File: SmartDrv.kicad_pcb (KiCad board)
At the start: 4 copper layers, 60 x 60 mm, 97 parts, among them J1 Conn_01x04, J2 Conn_01x02, J3 Conn_01x02, J4 Conn_01x02, J5 Conn_01x02, J6 Conn_01x02, J7 Conn_01x03, Q1 BSC040N10NS5, Q2 BSC040N10NS5, Q3 BSC040N10NS5, Q4 BSC040N10NS5, Q5 PMOS, Q6 NPN, U1 IR2104, U2 IR2104, U3 AT32F423CBT7, U4 MCP6002-xSN, U5 TJA1051T, U6 AMS1117-5.0, U7 AP2112K-3.3, U8 L7812, U9 KF7.62-2P, Y1 Crystal_GND24

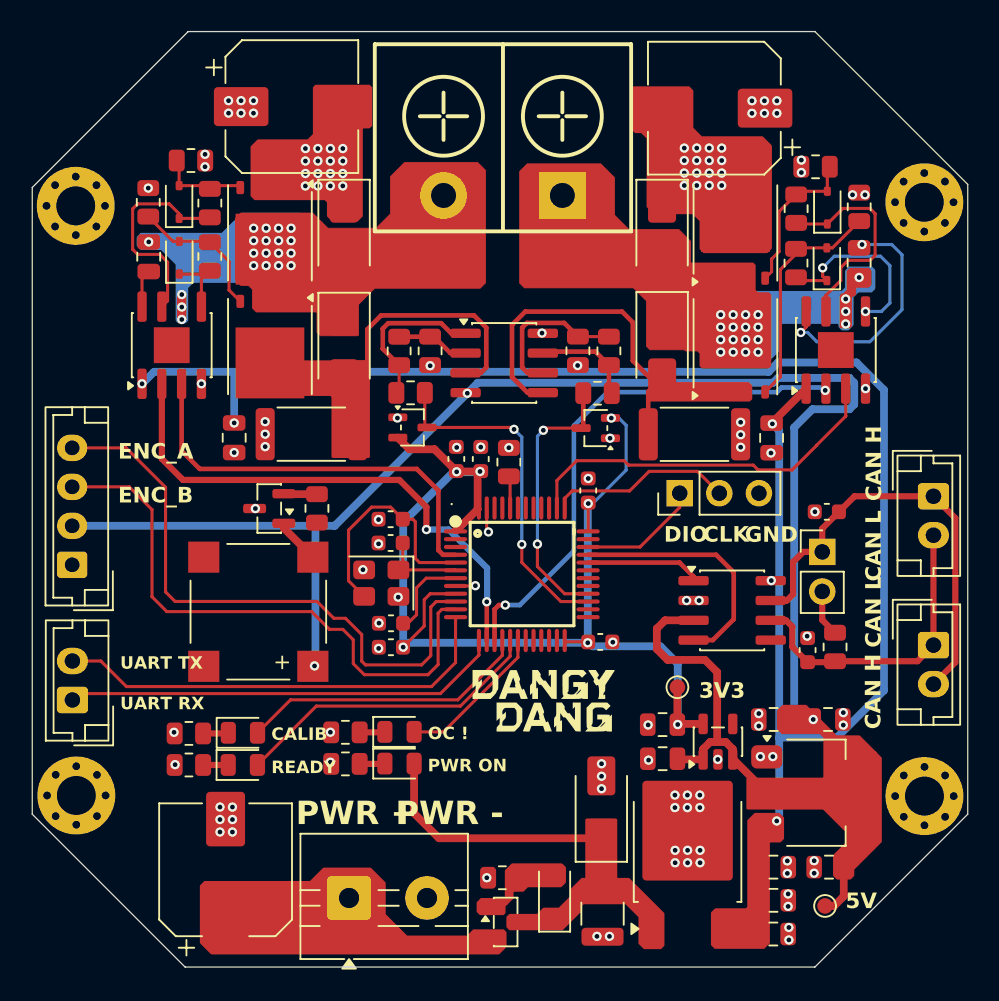
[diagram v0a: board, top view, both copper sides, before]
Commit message: Add files via upload
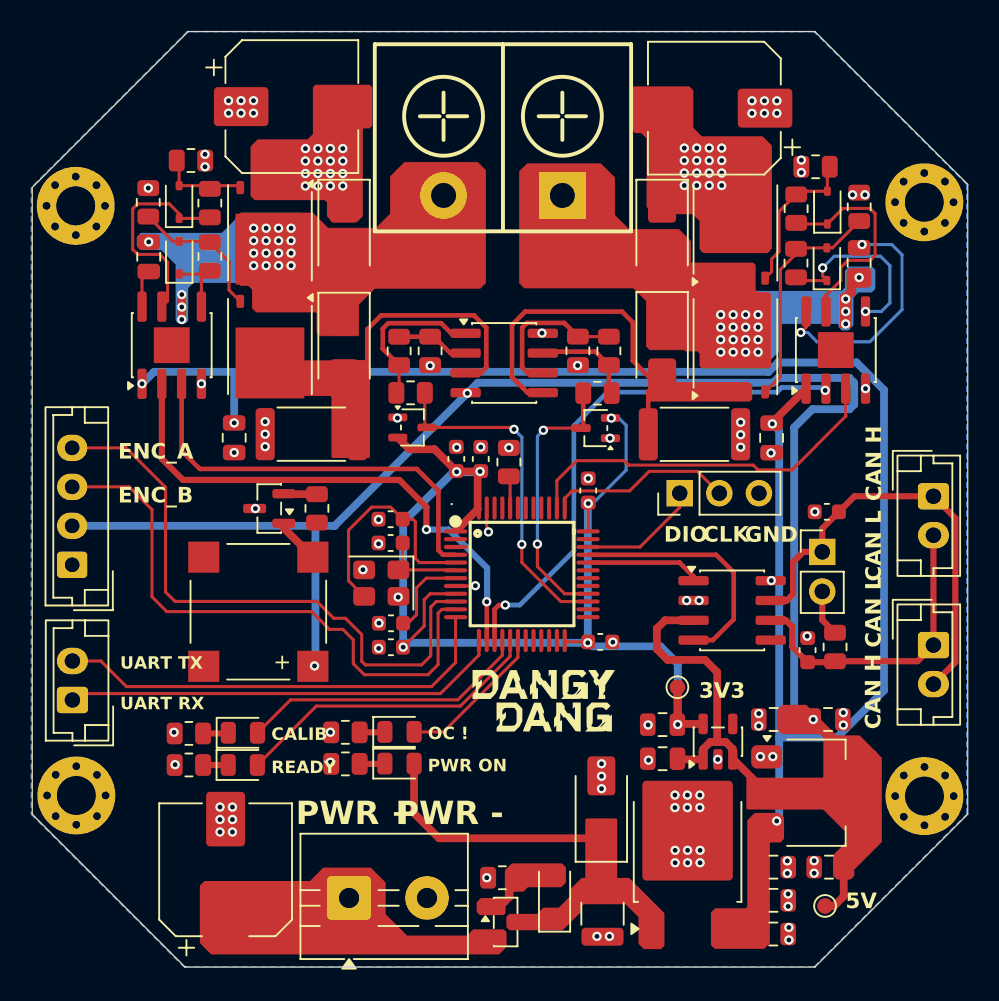
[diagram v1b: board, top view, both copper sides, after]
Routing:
- added copper zone on B.Cu, net GND
- added copper zone on In1.Cu, net V_IN
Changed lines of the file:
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@@
+		(net 4)
+		(net_name "GND")
+		(layer "B.Cu")
+		(hatch edge 0.5)
+		(connect_pads yes
+			(clearance 0.5)
+		)
+		(min_thickness 0.25)
+		(filled_areas_thickness no)
+		(fill yes
+			(thermal_gap 0.5)
+			(thermal_bridge_width 0.5)
+		)
+		(polygon
+			(pts
+				(xy 209.833 27.485) (xy 199.831 37.487) (xy 199.831 77.685) (xy 209.635 87.489) (xy 250.033 87.489)
+				(xy 259.83 77.692) (xy 259.83 37.291) (xy 250.024 27.485)
+			)
+		)
+	)
+	(zone
+		(net 49)
+		(net_name "V_IN")
+		(layer "In1.Cu")
+		(hatch edge 0.5)
+		(connect_pads yes
+			(clearance 0.5)
+		)
+		(min_thickness 0.25)
+		(filled_areas_thickness no)
+		(fill yes
+			(thermal_gap 0.5)
+			(thermal_bridge_width 0.5)
+		)
+		(polygon
+			(pts
+				(xy 209.803 27.485) (xy 199.801 37.487) (xy 199.801 77.685) (xy 209.605 87.489) (xy 250.003 87.489)
+				(xy 259.8 77.692) (xy 259.8 37.291) (xy 249.994 27.485)
+			)
+		)
+	)
+	(zone
 		(net 4)
 		(net_name "GND")
@@
 		(layer "In2.Cu")
 		(hatch edge 0.5)
-		(priority 1)
-		(connect_pads
+		(connect_pads yes
 			(clearance 0.5)
 		)
@@
 		(polygon
 			(pts
-				(xy 209.91 27.47) (xy 209.72 87.5) (xy 250.08 87.5) (xy 250.09 87.49) (xy 250.09 27.51) (xy 250.05 27.47)
-				(xy 209.9 27.47)
+				(xy 209.83 27.485) (xy 199.828 37.487) (xy 199.828 77.685) (xy 209.632 87.489) (xy 250.03 87.489)
+				(xy 259.827 77.692) (xy 259.827 37.291) (xy 250.021 27.485)
 			)
 		)

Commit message: Add files via upload
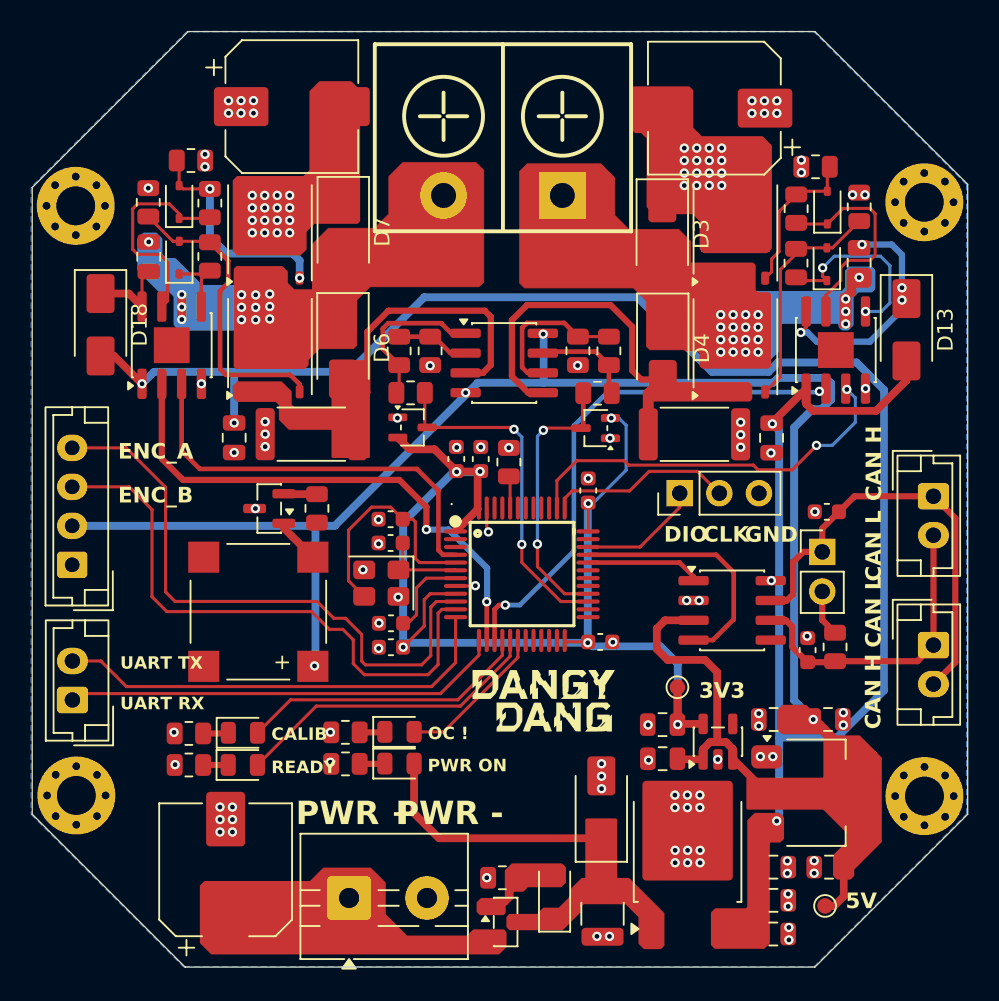
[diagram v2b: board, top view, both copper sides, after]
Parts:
- added D13: SS110, Diode_SMD:D_SMA, F.Cu at (256.0, 46.6)
- added D18: SS110, Diode_SMD:D_SMA, F.Cu at (204.3, 46.3)
- D15: value SMAJ6.0A -> SMAJ30.0A
- D3, D4, D6, D7: value 1N5819 -> SS310
- R12: value 20k -> 15k
- R22, R23, R24, R25: value 10 -> 1M
- moved D6 20.5 mm to (219.8, 47.8)
- moved D3 20.4 mm to (240.3, 40.5)
- moved D7 7.43 mm to (219.8, 40.3)
- moved D4 7.30 mm to (240.3, 47.8)
- turned Q2 to 90 degrees
- turned Q3 to 90 degrees
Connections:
- C8 pad 2: Net-(D4-A) -> Net-(D3-A)
- C9 pad 2: Net-(D3-A) -> Net-(D6-K)
- D4 pad 1: V_IN -> Net-(D3-A)
- D4 pad 2: Net-(D4-A) -> R_shunt_1
- D6 pad 1: Net-(D4-A) -> Net-(D6-K)
- D6 pad 2: R_shunt_1 -> R_shunt_2
- D7 pad 1: Net-(D3-A) -> V_IN
- D7 pad 2: R_shunt_2 -> Net-(D6-K)
- Q1 pad 1: Net-(D4-A) -> Net-(D3-A)
- Q1 pad 2: Net-(D4-A) -> Net-(D3-A)
- Q1 pad 3: Net-(D4-A) -> Net-(D3-A)
- Q2 pad 1: V_IN -> Net-(D6-K)
- Q2 pad 2: V_IN -> Net-(D6-K)
- Q2 pad 3: V_IN -> Net-(D6-K)
- Q2 pad 5: Net-(D3-A) -> V_IN
- Q3 pad 1: Net-(D3-A) -> R_shunt_2
- Q3 pad 2: Net-(D3-A) -> R_shunt_2
- Q3 pad 3: Net-(D3-A) -> R_shunt_2
- Q3 pad 5: R_shunt_2 -> Net-(D6-K)
- Q4 pad 5: Net-(D4-A) -> Net-(D3-A)
- U1 pad 6: Net-(D4-A) -> Net-(D3-A)
- U2 pad 6: Net-(D3-A) -> Net-(D6-K)
- U4 pad 4: +5V -> GND
- U4 pad 8: GND -> +5V
- U9 pad 1: Net-(D4-A) -> Net-(D3-A)
- U9 pad 2: Net-(D3-A) -> Net-(D6-K)
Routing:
- net +12V: track 108.3 -> 125.3 mm
- net Net-(D9-A): track 9.23 -> 19.4 mm
- net Net-(D2-A): track 5.64 -> 14.3 mm, vias 0 -> 2
- net Net-(D18-K): track 2.43 -> 5.44 mm
- net R_shunt_2: track 17.0 -> 19.0 mm
- net EN1: track 24.3 -> 25.3 mm, vias 0 -> 2
- net +5V: track 113.6 -> 112.8 mm
- net R_shunt_1: track 22.9 -> 23.6 mm
- net Net-(D6-K): vias 0 -> 13
- net Net-(D4-A): vias 20 -> 0
- net Net-(D13-K): vias 2 -> 4
